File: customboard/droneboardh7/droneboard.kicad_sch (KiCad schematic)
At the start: 62 parts, among them J1 Conn_01x04, J10 Conn_01x03_Pin, J2 Conn_01x04, J3 Conn_01x05_Pin, J4 Conn_01x02_Pin, J5 USB_C_Receptacle_USB2.0_16P, J6 Conn_01x04, SW1 SW_Push, SW2 SW_Push, U1 AP62300Z6, U2 STM32H723VGTx, U4 ICM-42688-P, U5 SPX3819M5-L-3-3, U6 SPX3819M5-L-3-3, Y2 CSTNE20M0V53Z000R0

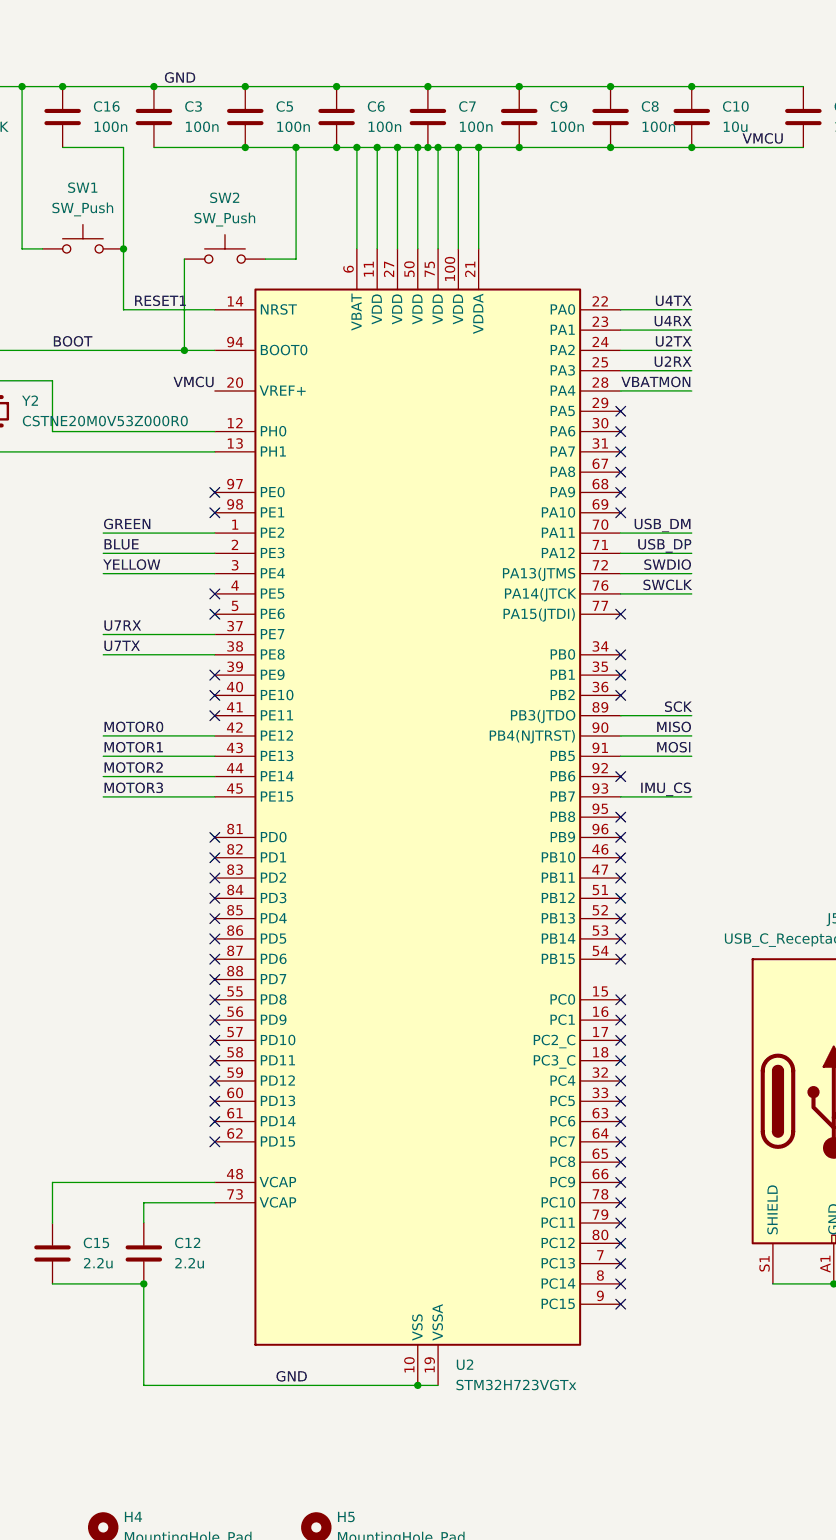
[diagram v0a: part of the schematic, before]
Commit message: stuff
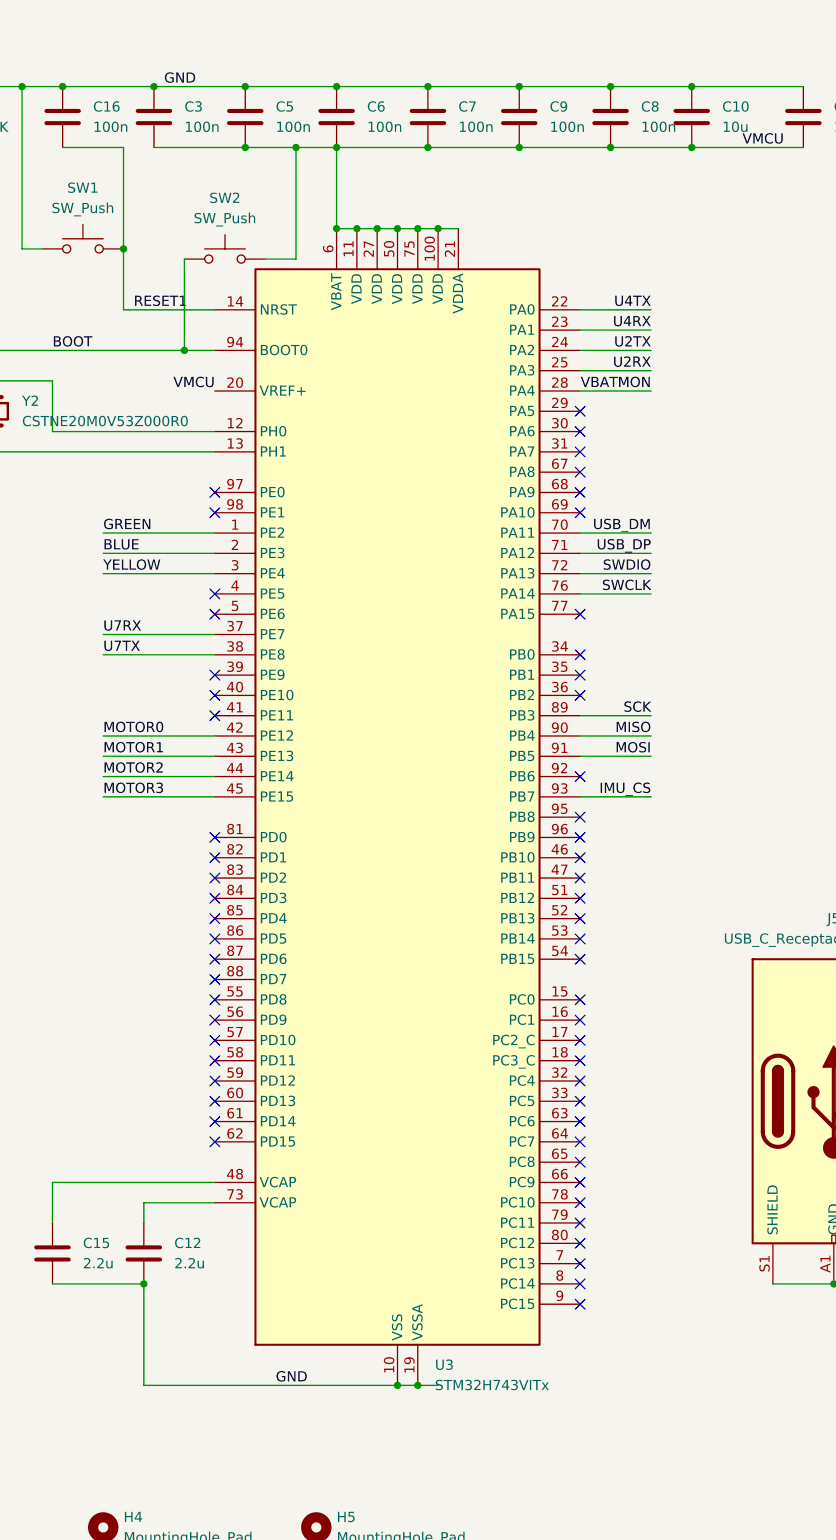
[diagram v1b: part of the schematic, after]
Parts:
- removed U2: STM32H723VGTx, Package_QFP:LQFP-100_14x14mm_P0.5mm, symbol MCU_ST_STM32H7:STM32H723VGTx
- added U3: STM32H743VITx, Package_QFP:LQFP-100_14x14mm_P0.5mm, symbol MCU_ST_STM32H7:STM32H743VITx
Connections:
- net BLUE: now also U3.2 (PE3)
- net BOOT: now also U3.94 (BOOT0)
- net GND: now also U3.10 (VSS), U3.19 (VSSA), U3.26 (VSS), U3.49 (VSS), U3.74 (VSS), U3.99 (VSS)
- net GREEN: now also U3.1 (PE2)
- net IMU_CS: now also U3.93 (PB7)
- net MISO: now also U3.90 (PB4)
- net MOSI: now also U3.91 (PB5)
- net MOTOR0: now also U3.42 (PE12)
- net MOTOR1: now also U3.43 (PE13)
- net MOTOR2: now also U3.44 (PE14)
- net MOTOR3: now also U3.45 (PE15)
- net RESET1: now also U3.14 (NRST)
- net SCK: now also U3.89 (PB3)
- net SWCLK: now also U3.76 (PA14)
- net SWDIO: now also U3.72 (PA13)
- net U2RX: now also U3.25 (PA3)
- net U2TX: now also U3.24 (PA2)
- net U4RX: now also U3.23 (PA1)
- net U4TX: now also U3.22 (PA0)
- net U7RX: now also U3.37 (PE7)
- net U7TX: now also U3.38 (PE8)
- net USB_DM: now also U3.70 (PA11)
- net USB_DP: now also U3.71 (PA12)
- net VBATMON: now also U3.28 (PA4)
- net VMCU: now also U3.100 (VDD), U3.11 (VDD), U3.20 (VREF+), U3.21 (VDDA), U3.27 (VDD), U3.50 (VDD), U3.6 (VBAT), U3.75 (VDD)
- net YELLOW: now also U3.3 (PE4)
- net at Y2.1: now also U3.12 (PH0)
- net at Y2.3: now also U3.13 (PH1)
- net at C12.1: now also U3.73 (VCAP)
- net at C15.1: now also U3.48 (VCAP)
